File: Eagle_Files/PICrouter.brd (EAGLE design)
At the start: 104.7 x 33.3 mm, 77 parts, among them IC1 PIC32MX675F512H, IC2 48M033F, IC3 DP83848, J1 POWER_JACK, J3 POWER_JACK, Q1 20MHz, X2 USB_B

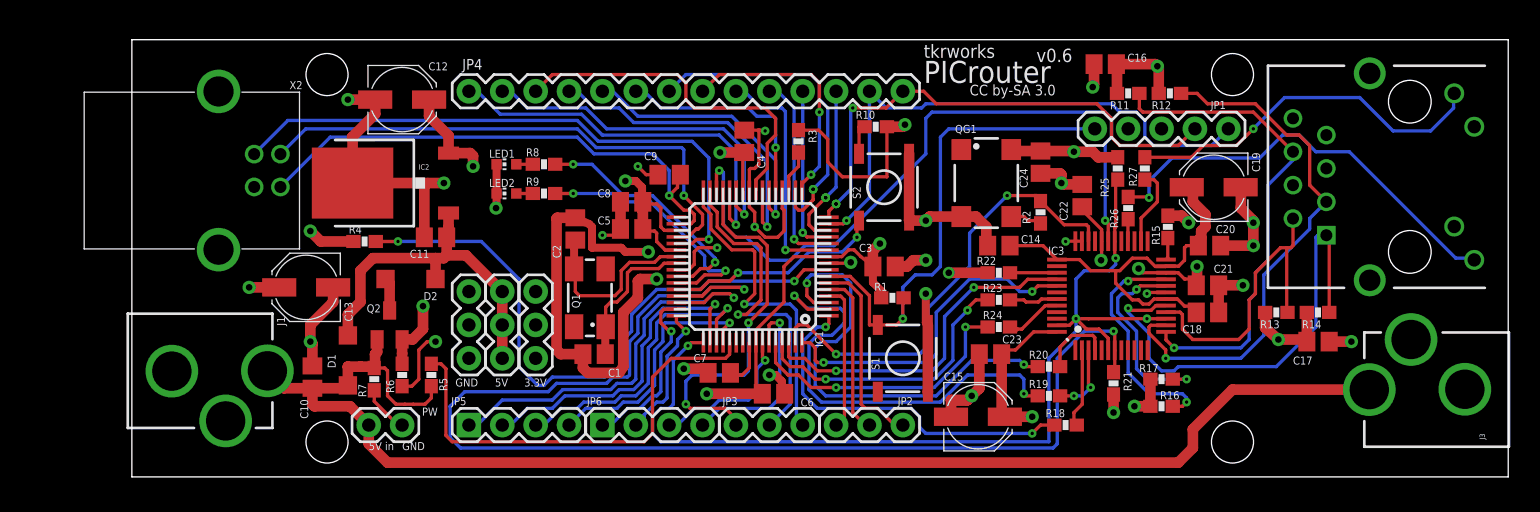
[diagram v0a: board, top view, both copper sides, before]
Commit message: Released PICrouter schematic and board v0.71.
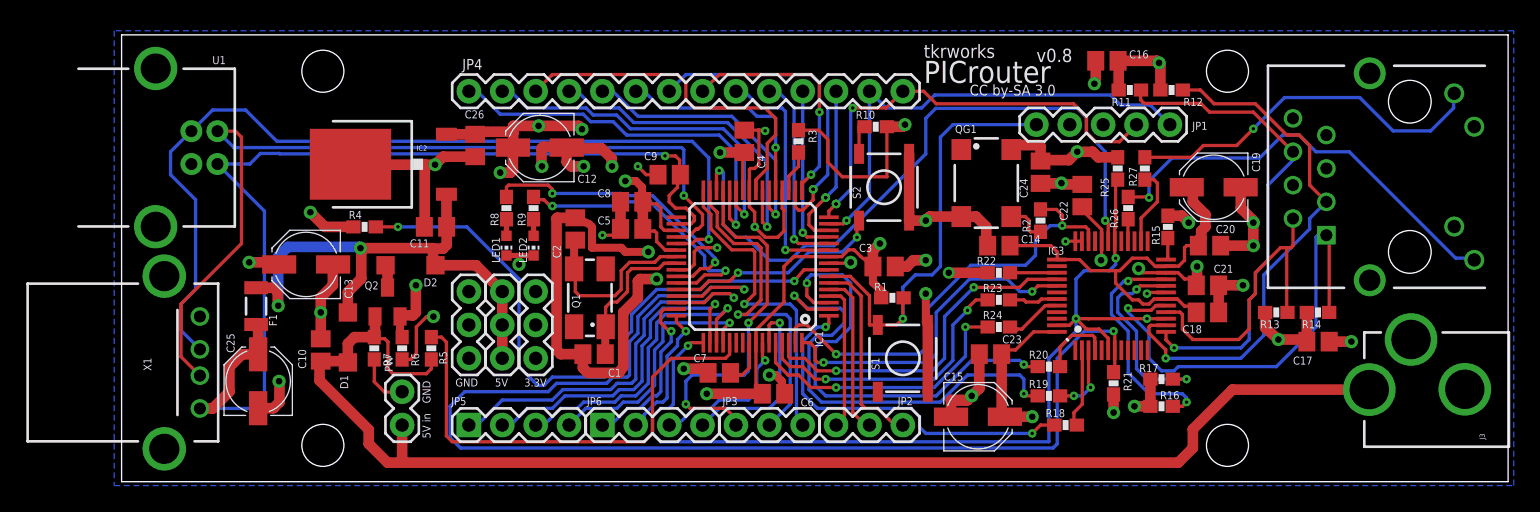
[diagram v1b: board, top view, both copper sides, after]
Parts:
- removed J1: POWER_JACK, SparkFun:POWER_JACK_PTH_LOCK
- removed X2: USB_B, con-cypressindustries:85-32004-10X
- added C25: 100uF, rcl:PANASONIC_C
- added C26: 0.1uF, rcl:C2012
- added F1: PTCSMD, SparkFun:PTC-1206
- added U1: USB+SHIELD, SparkFun:USB-B-PTH
- added X1: USB-A-H, SparkFun:USB-A-H
- IC1: device PIC:TQFP64-10X10 -> PIC.rpt:TQFP64-10X10
- moved C12 11.1 mm to (31.1, 25.1), turned to 180 degrees
- moved LED1 6.19 mm to (28.6, 17.6), turned to 180 degrees
- moved LED2 4.47 mm to (30.6, 17.6), turned to 180 degrees
- moved JP1 4.46 mm to (68.9, 26.8)
- moved R8 4.39 mm to (28.6, 20.5), turned to 90 degrees
- moved PW 2.54 mm to (20.6, 3.97), turned to 90 degrees
- moved R7 2.35 mm to (18.5, 9.81)
- moved C10 2.16 mm to (14.4, 9.68)
- moved R5 2.03 mm to (22.9, 9.81)
- moved R6 2.03 mm to (20.6, 9.81)
- moved Q2 1.75 mm to (19.5, 13.3)
- moved C13 1.75 mm to (13.3, 16.2)
- moved D1 1.75 mm to (16.5, 10.6)
- moved IC2 1.44 mm to (19.2, 23.8)
- moved R9 1.37 mm to (30.6, 20.5), turned to 90 degrees
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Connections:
- removed net N$61: C13.+, C9.2, IC1.34, Q2.2, R4.1, R6.2, X2.1
- new net N$50: C13.+, C25.+, C9.2, F1.1, IC1.34, Q2.2, R4.1, R6.2, U1.VBUS, X1.VBUS
- net GND: now also C25.-, C26.2, U1.GND, U1.S1, U1.S2, X1.GND, X1.GND2, X1.GND3; no longer J1.GND, X2.4
- net N$45: now also U1.D-, X1.D-; no longer X2.2
- net N$46: no longer J1.PWR
- net N$5: now also U1.D+, X1.D+; no longer X2.3
- net VCC: now also F1.2
- net VDD: now also C26.1
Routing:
- net N$50: track 0.00 -> 117.7 mm, vias 0 -> 4
- net N$61: track 76.6 -> 0.00 mm, vias 4 -> 0
- net N$45: track 40.8 -> 67.4 mm
- net N$5: track 45.6 -> 69.5 mm
- net VCC: track 27.6 -> 41.4 mm, vias 0 -> 2
- net VDD: track 121.6 -> 130.9 mm, vias 16 -> 18
- net N$3: track 42.6 -> 36.8 mm
- net N$4: track 38.7 -> 34.0 mm
- net N$6: track 38.0 -> 33.7 mm
- net N$51: track 0.00 -> 4.13 mm
- net N$13: track 18.8 -> 22.9 mm
- net N$44: track 0.00 -> 3.35 mm
- net N$46: track 107.7 -> 105.6 mm
- net N$11: track 34.3 -> 36.3 mm
- net N$14: track 20.0 -> 21.8 mm
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- added copper zone on layer 16, net GND
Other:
- board size 104.7 x 33.3 mm -> 105.5 x 34 mm
- board text added: "v0.8"
- board text removed: "v0.6"

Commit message: Released PICrouter schematic and board v0.8.
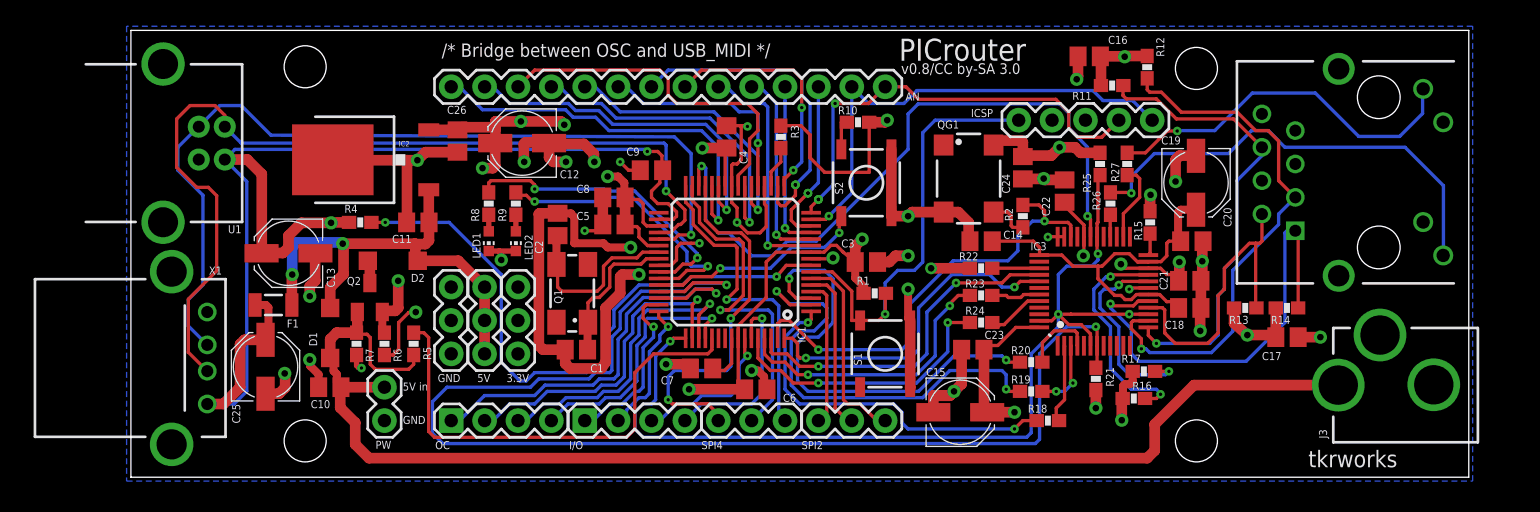
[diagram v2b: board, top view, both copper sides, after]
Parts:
- removed JP1: (no value), SparkFun:1X05
- removed JP2: SPI2, SparkFun:1X03
- removed JP3: SPI4, SparkFun:1X03
- removed JP4: AN, SparkFun:1X14
- removed JP5: OC, SparkFun:1X04
- removed JP6: I/O, SparkFun:1X04
- added AN: (no value), SparkFun:1X14
- added I/O, OC: (no value), SparkFun:1X04
- added ICSP: (no value), SparkFun:1X05
- added SPI2, SPI4: (no value), SparkFun:1X03
- C13: value 100uF -> 10uF
- C25: value 100uF -> 150uF
- U1: value USB+SHIELD -> DEVICE
- moved PW 3.18 mm to (19.3, 6.85), turned to 270 degrees
- moved C10 2.92 mm to (15.1, 6.85), turned to 180 degrees
- moved R12 2.54 mm to (77.3, 31.2), turned to 90 degrees
- moved J2 2.39 mm to (95.0, 23.2)
- moved C17 2.39 mm to (88.0, 10.7)
- moved J3 2.39 mm to (105.7, 7.01)
- moved R13 2.39 mm to (84.8, 12.9)
- moved R14 2.39 mm to (88.0, 12.9)
- moved R16 2.19 mm to (76.3, 5.99)
- moved C13 1.59 mm to (12.0, 17.0)
- moved R17 1.47 mm to (77.1, 8.06)
- moved C18 1.39 mm to (80.6, 12.9)
- moved C21 1.39 mm to (80.6, 14.9)
- moved R18 1.39 mm to (69.8, 4.31)
- moved R22 1.39 mm to (64.7, 15.9)
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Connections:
- net GND: now also ICSP.3; no longer JP1.3
- net N$18: now also AN.3; no longer JP4.3
- net N$19: now also AN.4; no longer JP4.4
- net N$20: now also AN.5; no longer JP4.5
- net N$21: now also AN.6; no longer JP4.6
- net N$22: now also AN.7; no longer JP4.7
- net N$23: now also AN.8; no longer JP4.8
- net N$24: now also AN.9; no longer JP4.9
- net N$25: now also AN.10; no longer JP4.10
- net N$26: now also AN.11; no longer JP4.11
- net N$27: now also AN.12; no longer JP4.12
- net N$28: now also AN.13; no longer JP4.13
- net N$29: now also AN.14; no longer JP4.14
- net N$3: now also AN.2, ICSP.5; no longer JP1.5, JP4.2
- net N$30: now also SPI2.1; no longer JP2.1
- net N$31: now also SPI2.2; no longer JP2.2
- net N$32: now also SPI2.3; no longer JP2.3
- net N$33: now also SPI4.2; no longer JP3.2
- net N$34: now also SPI4.3; no longer JP3.3
- net N$35: now also SPI4.1; no longer JP3.1
- net N$36: now also OC.1; no longer JP5.1
- net N$37: now also I/O.1; no longer JP6.1
- net N$38: now also OC.2; no longer JP5.2
- net N$39: now also OC.3; no longer JP5.3
- net N$4: now also AN.1, ICSP.4; no longer JP1.4, JP4.1
- net N$40: now also OC.4; no longer JP5.4
- net N$41: now also I/O.2; no longer JP6.2
- net N$42: now also I/O.3; no longer JP6.3
- net N$43: now also I/O.4; no longer JP6.4
- net N$6: now also ICSP.1; no longer JP1.1
- net VDD: now also ICSP.2; no longer JP1.2
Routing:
- net N$50: track 117.7 -> 106.7 mm, vias 4 -> 3
- net GND: track 169.5 -> 164.6 mm, vias 33 -> 35
- net VCC: track 41.4 -> 36.7 mm
- net N$45: track 67.4 -> 70.6 mm
- net N$55: track 33.0 -> 35.1 mm
- net RDM: track 37.1 -> 35.1 mm
- net N$5: track 69.5 -> 67.5 mm
- net PFBOUT: track 31.0 -> 29.4 mm
- net TDP: track 35.7 -> 34.4 mm
- net N$12: track 49.1 -> 48.1 mm
- net N$47: track 17.9 -> 17.1 mm
- net VDD: track 130.9 -> 130.2 mm
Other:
- board size 105.5 x 34 mm -> 101.8 x 34 mm
- board text added: "/* Bridge between OSC and USB_MIDI */"
- board text added: "HOST"
- board text added: "v0.8/CC by-SA 3.0"
- board text removed: "CC by-SA 3.0"
- board text removed: "v0.8"
